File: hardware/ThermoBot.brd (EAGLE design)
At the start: 91.4 x 53.3 mm, 34 parts, among them U1 VSK-S5, U2 MAX31856, U3 LTV-354T, U4 FODM3053, U5 T25

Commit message: Renamed to ThermoBot
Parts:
- AC/L, AC/N, HTR/L, HTR/N: device Tempatroller:QUICK-1 -> ThermoBot:QUICK-1
- AIO: device Tempatroller:1X06 -> ThermoBot:1X06
- C1: device Tempatroller:153CLV-1014 -> ThermoBot:153CLV-1014
- C2, C3, C4, C5, C6, C7: device Tempatroller:C0805 -> ThermoBot:C0805
- DIO-H: device Tempatroller:1X10 -> ThermoBot:1X10
- DIO-L, POWER: device Tempatroller:1X08 -> ThermoBot:1X08
- F1: device Tempatroller:2SMD-2410 -> ThermoBot:2SMD-2410
- JP1, JP3: device Tempatroller:SCREWTERMINAL-5MM-2 -> ThermoBot:SCREWTERMINAL-5MM-2
- LED1, LED2, LED3: device Tempatroller:CHIP-LED0805 -> ThermoBot:CHIP-LED0805
- R1, R2, R4: device Tempatroller:R1206 -> ThermoBot:R1206
- R3, R5, R6, R7: device Tempatroller:R0805 -> ThermoBot:R0805
- U$1: device Tempatroller:SILK_QC -> ThermoBot:SILK_QC
- U1: device Tempatroller:VSK-S5 -> ThermoBot:VSK-S5
- U2: device Tempatroller:TSSOP14 -> ThermoBot:TSSOP14
- U3, U4: device Tempatroller:SOP-4 -> ThermoBot:SOP-4
- U5: device Tempatroller:TO263-3 -> ThermoBot:TO263-3

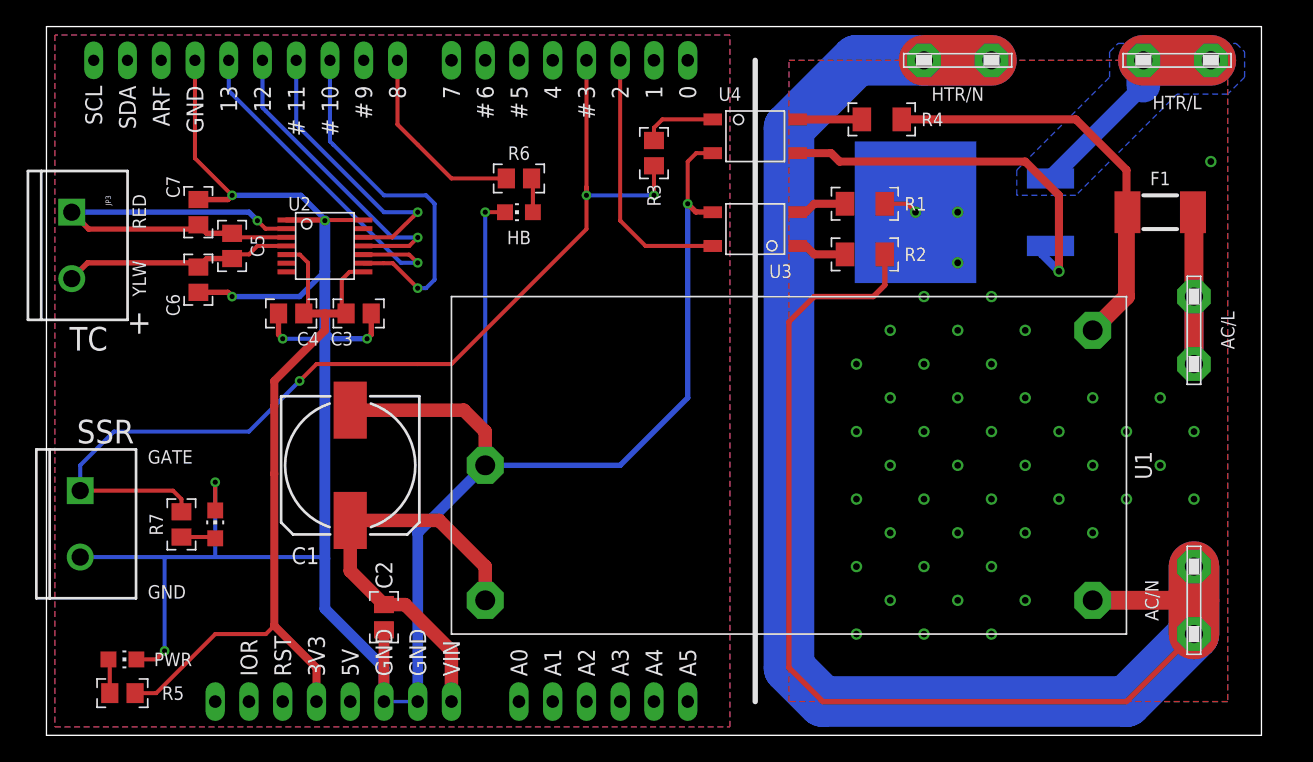
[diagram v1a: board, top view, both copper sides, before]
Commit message: Started hardware revisions for v1B
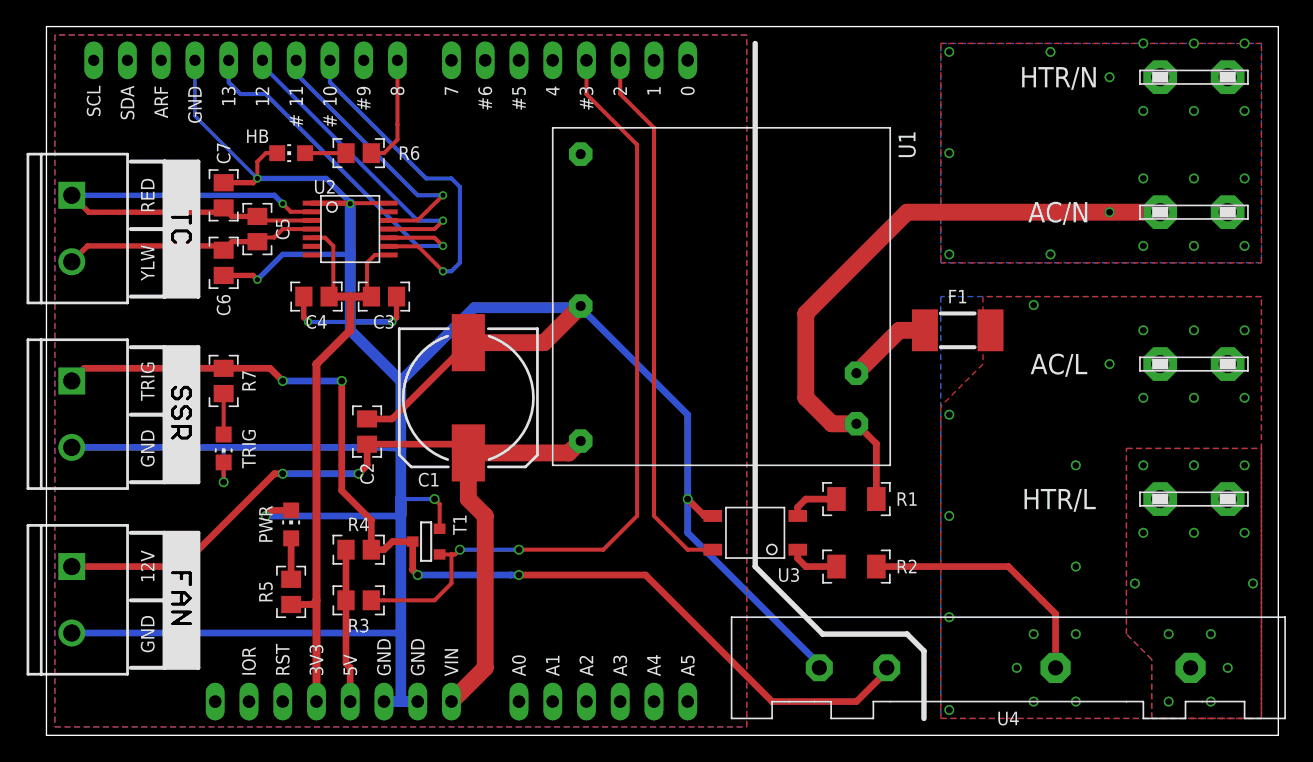
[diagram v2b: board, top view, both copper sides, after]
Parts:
- removed U5: T25, ThermoBot:TO263-3
- added JP2: M025MM, ThermoBot:SCREWTERMINAL-5MM-2
- added T1: (no value), SmslsTron:SOT-23
- added U$2: (no value), ThermoBot:SILK_FAN
- added U$3: (no value), ThermoBot:SILK_SSR
- added U$4: (no value), ThermoBot:SILK_TC
- R3: value 100 -> 10k
- R4: value 1k -> 100; device ThermoBot:R1206 -> ThermoBot:R0805
- U1: value VSK-S5 -> AC/DC-CONV-ECE05US12; device ThermoBot:VSK-S5 -> ThermoBot:ECE05
- U4: value FODM3053 -> SSR-PF240D25R; device ThermoBot:SOP-4 -> ThermoBot:SIP-4
- moved R4 51.0 mm to (23.5, 14.0), turned to 180 degrees
- moved U4 44.3 mm to (72.4, 5.08)
- moved R3 40.3 mm to (23.5, 10.2), turned to 180 degrees
- moved HTR/L 33.0 mm to (86.4, 17.8)
- moved AC/N 29.2 mm to (86.4, 39.4), turned to 180 degrees
- moved R2 23.5 mm to (61.0, 12.7)
- moved U3 22.9 mm to (53.3, 15.2)
- moved R1 22.2 mm to (61.0, 17.8)
- moved HTR/N 17.8 mm to (86.4, 49.5), turned to 180 degrees
- moved LED2 17.7 mm to (18.4, 43.8)
- moved F1 17.6 mm to (68.6, 30.5)
- moved LED1 16.3 mm to (18.4, 15.9), turned to 270 degrees
- moved R5 14.8 mm to (18.4, 10.8), turned to 90 degrees
- moved C2 14.0 mm to (24.1, 22.9), turned to 90 degrees
- moved U1 13.7 mm to (50.8, 33.0)
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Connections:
- removed net N$1: R4.1, U4.4
- removed net N$2: R3.2, U4.1
- removed net N$5: U4.3, U5.2
- new net HTR_TRIG: JP1.1, R4.1, R7.1, T1.1, U4.DC+
- net +5V: now also R3.2, R4.2
- net AC/L: now also R2.1, U4.AC2; no longer R1.1, U5.3
- net AC/L-F: no longer R4.2
- net AC/N: now also R1.1; no longer R2.1
- net GND: now also JP2.2, T1.2, U4.DC-; no longer U4.2
- net HTR/L: now also U4.AC1; no longer U5.1
- net HTR_SIG/D3: now also T1.3; no longer JP1.1, R7.1
- net VIN: now also JP2.1, U1.5; no longer U1.3
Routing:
- net AC/N: track 187.4 -> 47.1 mm, vias 0 -> 19
- net HTR_TRIG: track 0.00 -> 81.2 mm, vias 0 -> 4
- net VIN: track 31.9 -> 64.0 mm, vias 0 -> 2
- net N$5: track 29.4 -> 0.00 mm, vias 1 -> 0
- net AC/L-F: track 31.7 -> 6.49 mm
- net HTR/L: track 21.9 -> 0.00 mm, vias 0 -> 13
- net AC_ZC/D2: track 19.8 -> 40.8 mm
- net HTR_SIG/D3: track 76.8 -> 60.7 mm, vias 3 -> 2
- net GND: track 223.9 -> 238.5 mm
- net +5V: track 0.00 -> 11.6 mm
- net +3V3: track 58.2 -> 47.1 mm
- net HB/D8: track 14.7 -> 8.36 mm
- net N$2: track 5.64 -> 0.00 mm
- net AC/L: track 24.3 -> 19.0 mm, vias 47 -> 19
- net N$1: track 4.83 -> 0.00 mm
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- added copper zone on layer 1, net AC/N
- added copper zone on layer 16, net AC/N
- added copper zone on layer 1, net HTR/L
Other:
- board size 91.4 x 53.3 mm -> 92.7 x 53.3 mm
- board text removed: "+"
- board text removed: "GATE"
- board text removed: "RED"
- board text removed: "SSR"
- board text removed: "TC"
- board text removed: "YLW"
